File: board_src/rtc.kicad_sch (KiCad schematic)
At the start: 7 parts, among them IC1 PCF8563TS_4,118, J10 Conn_01x02_Pin, J9 Conn_01x02_Pin, Y2 Crystal

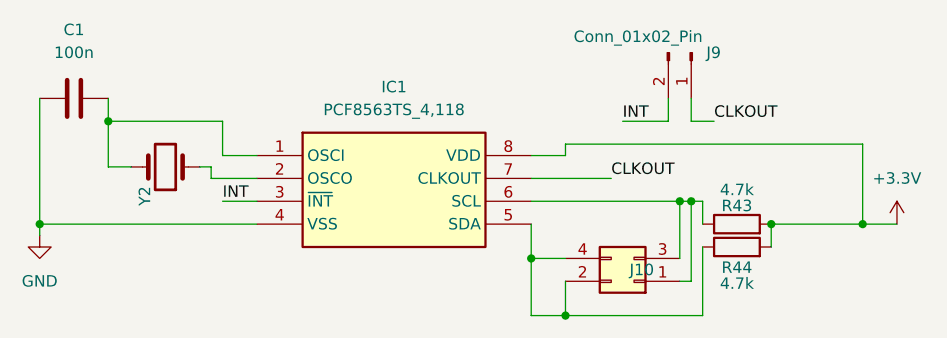
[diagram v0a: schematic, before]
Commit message: sciezki polaczen
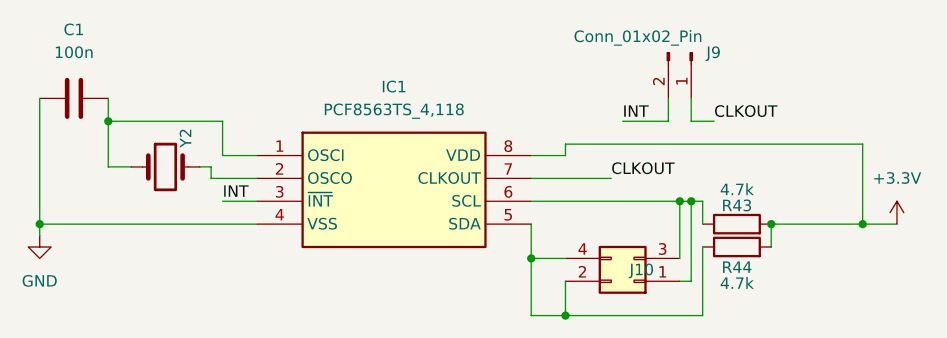
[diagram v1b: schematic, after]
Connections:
- net at C1.2, IC1.1 (OSCI): now also Y2.1; no longer Y2.2
- net at IC1.2 (OSCO): now also Y2.2; no longer Y2.1
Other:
- moved on the sheet: Y2
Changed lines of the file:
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@@
 	(symbol
 		(lib_id "Device:Crystal")
-		(at 176.53 76.2 180)
+		(at 176.53 76.2 0)
 		(unit 1)
 		(exclude_from_sim no)
@@
 		(dnp no)
 		(property "Reference" "Y2"
-			(at 174.244 80.518 90)
+			(at 178.816 71.882 90)
 			(effects
 				(font
@@
 		)
 		(property "Value" "Crystal"
-			(at 178.816 73.152 90)
+			(at 174.244 79.248 90)
 			(effects
 				(font
